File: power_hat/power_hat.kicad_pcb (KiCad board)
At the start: 4 copper layers, 47.1 x 133.6 mm, 49 parts, among them IC1 TPS259830LNRGER, IC2 INA238AQDGSRQ1, J1 XT30PW-M/Terminal block, J10 XT30PW-M/Terminal block, J11 XT30PW-M/Terminal block, J12 XT30PW-M/Terminal block, J13 502585-0570, J14 502585-0570, J2 XT30PW-M/Terminal block, J3 XT30PW-M/Terminal block, J4 XT30PW-M/Terminal block, J5 Conn_01x02_Pin, J6 XT30PW-M/Terminal block, J7 Conn_01x02_Pin, J8 XT30PW-M/Terminal block, J9 XT30PW-M/Terminal block, Q1 CSD18540Q5B

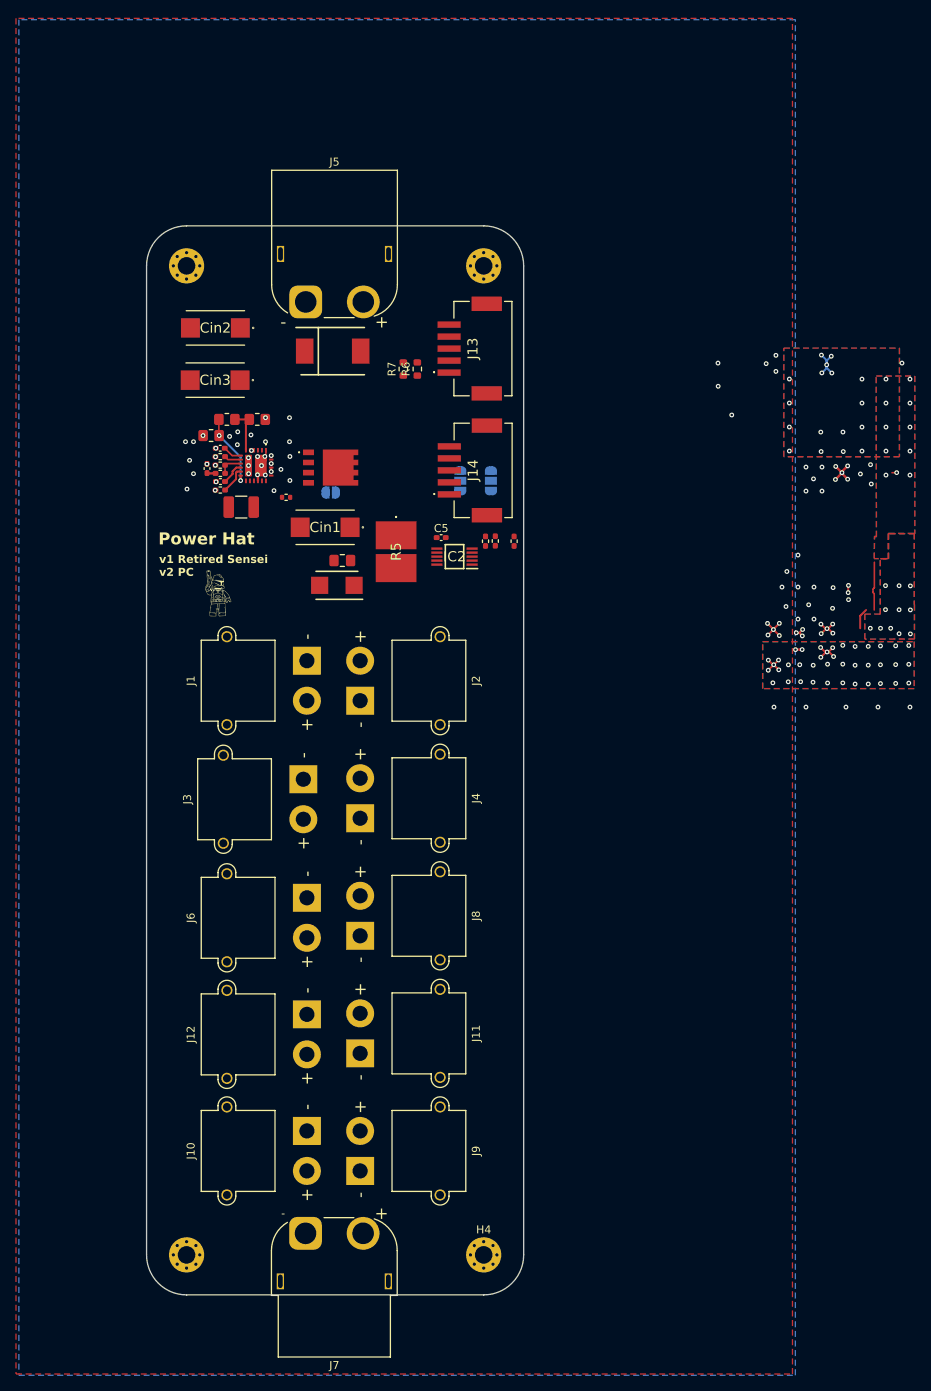
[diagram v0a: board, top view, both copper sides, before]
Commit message: Reruted a while ago with TPS, resized TPS with personal notes and Excel, issues with 24V one
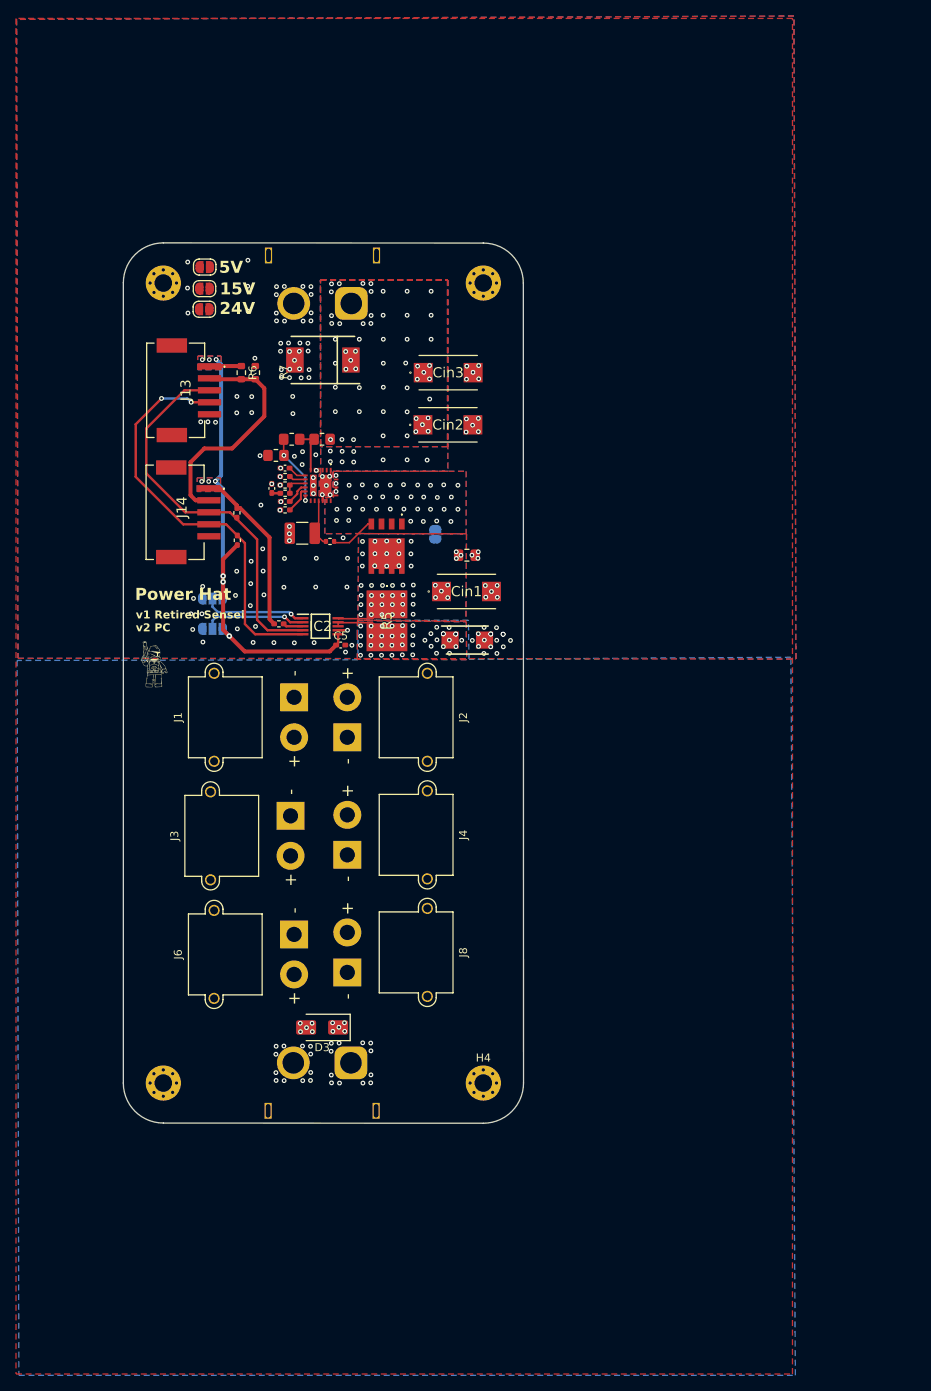
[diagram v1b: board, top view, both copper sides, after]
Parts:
- removed J10, J11, J12, J9: XT30PW-M/Terminal block, 0_connectors:AMASS_XT30PW-M_1x02_P2.50mm_Horizontal
- added D3: SMCJ28A, Diode_SMD:D_SMA, F.Cu at (83.2, 146.7)
- added JP4: Jumper_2_Open, Jumper:SolderJumper-2_P1.3mm_Open_RoundedPad1.0x1.5mm, F.Cu at (68.6, 51.6)
- added JP5: Jumper_2_Open, Jumper:SolderJumper-2_P1.3mm_Open_RoundedPad1.0x1.5mm, F.Cu at (68.5, 54.4)
- added JP6: Jumper_2_Open, Jumper:SolderJumper-2_P1.3mm_Open_RoundedPad1.0x1.5mm, F.Cu at (68.5, 56.9)
- J5, J7: moved to B.Cu
- moved J14 38.3 mm to (65.2, 82.3), turned to -90 degrees
- moved J13 38.2 mm to (65.2, 67.1), turned to -90 degrees
- moved JP3 37.8 mm to (69.5, 93.1), turned to 0 degrees
- moved JP2 36.1 mm to (69.5, 96.9), turned to 180 degrees
- moved R11 32.5 mm to (72.6, 82.4), turned to -90 degrees
- moved Cin2 31.5 mm to (99.0, 71.4), turned to 0 degrees
- moved R10 31.2 mm to (77.8, 96.2), turned to 180 degrees
- moved R12 31.0 mm to (72.7, 85.8), turned to 90 degrees
- moved Cin3 29.1 mm to (99.0, 64.8), turned to 0 degrees
- moved J7 22.1 mm to (86.8, 151.1), turned to 0 degrees
- moved R6 22.0 mm to (73.2, 64.8), turned to -90 degrees
- moved H2 21.7 mm to (63.4, 153.6)
- moved H4 21.5 mm to (103.4, 153.6)
- moved Cin1 19.4 mm to (101.3, 92.2), turned to 0 degrees
- moved IC2 18.9 mm to (83.0, 96.5), turned to 0 degrees
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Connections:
- IC2 pad 10: VCC -> /VOUT
- IC2 pad 8: /VOUT -> VCC
- IC2 pad 9: /VOUT -> VCC
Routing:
- net +3V3: track 0.00 -> 85.8 mm, vias 0 -> 9
- net /SCL: track 0.00 -> 52.3 mm, vias 0 -> 2
- net /SDA: track 0.00 -> 49.2 mm
- net /ID: track 0.00 -> 29.2 mm
- net GND: track 16.5 -> 2.54 mm, vias 72 -> 145
- net /A1: track 0.00 -> 13.0 mm, vias 0 -> 1
- net /A0: track 0.00 -> 12.8 mm, vias 0 -> 1
- net /VOUT: track 0.00 -> 6.86 mm, vias 0 -> 47
- net EFUSE: track 11.3 -> 5.38 mm, vias 37 -> 69
- net Net-(Q1-G): track 2.59 -> 5.69 mm
- net /ALERT: track 0.00 -> 2.53 mm
- net VCC: track 8.53 -> 7.38 mm, vias 39 -> 57
- net Net-(IC1-DVDT/_BGATE): track 6.10 -> 6.75 mm
- net /Efuse_out: vias 18 -> 36
- added copper zone on B.Cu, net +3V3
- added copper zone on F.Cu, net +3V3
- added copper zone on B.Cu, net /VOUT
- added copper zone on F.Cu, net /VOUT
- added copper zone on B.Cu, net GND
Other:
- board size 47.1 x 133.6 mm -> 50 x 110 mm
- board text added: "15V"
- board text added: "24V"
- board text added: "5V"
- board text added: "A0"
- board text added: "A1"
- board text added: "Address select"
- board text added: "Ok the Xt60 are put backwards because like this polarity is fixed"

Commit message: Rerouted and DRC repassed to put back ADM as TPS is thermally limited for 24V
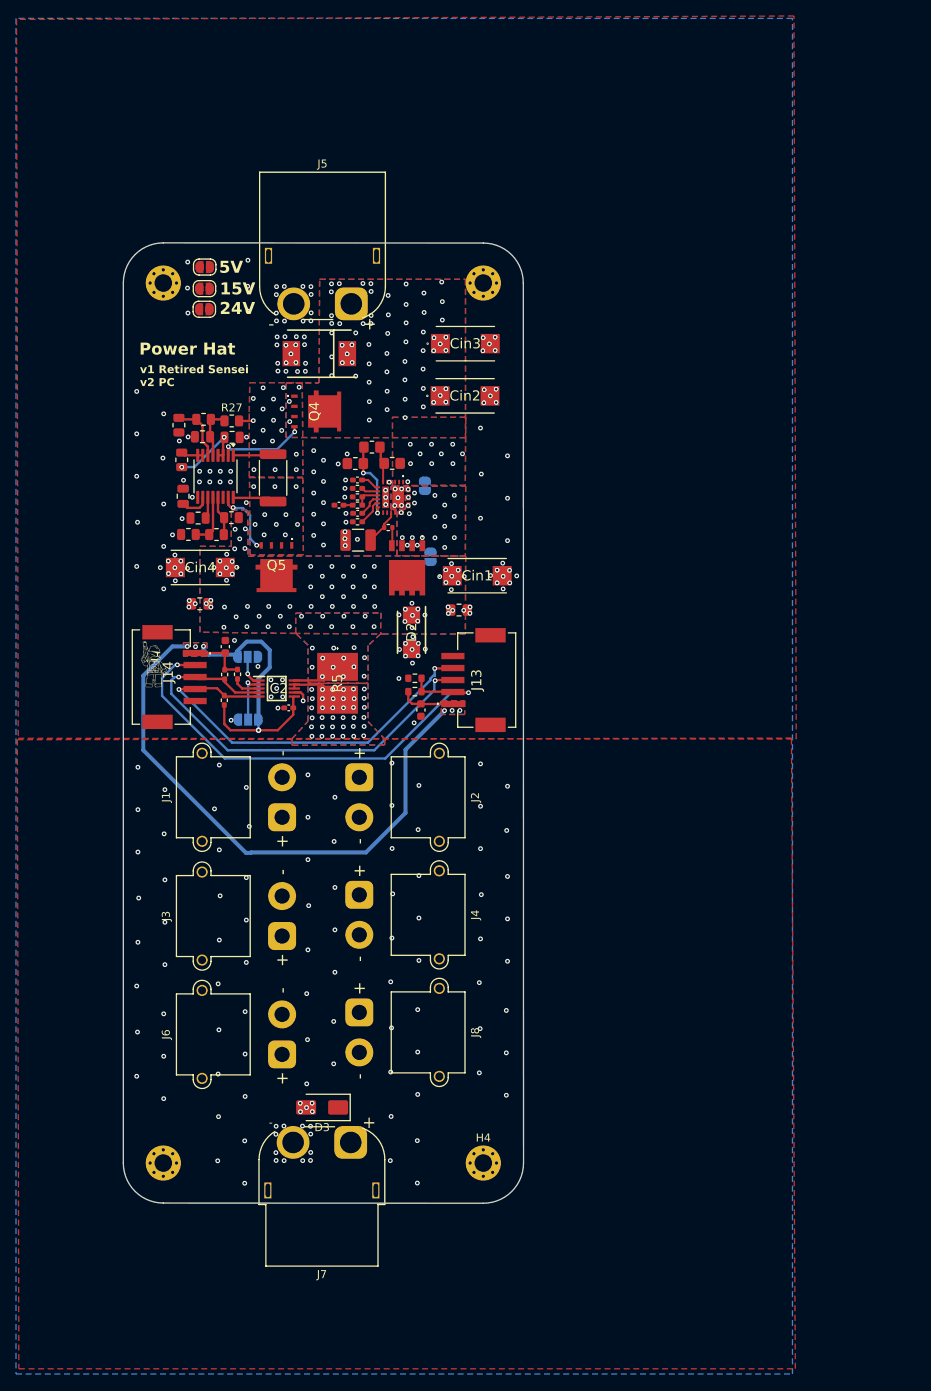
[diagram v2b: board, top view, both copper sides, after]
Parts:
- added C2: 1uF, Capacitor_SMD:C_0805_2012Metric_Pad1.18x1.45mm_HandSolder, F.Cu at (68.0, 93.7)
- added C3: 4u7 50V XR7, Capacitor_SMD:C_0603_1608Metric, F.Cu at (71.2, 99.1)
- added C38: 1uF - 50V X7R, Capacitor_SMD:C_0805_2012Metric, F.Cu at (72.0, 72.9)
- added C39: 1nF - 50V X7R, Capacitor_SMD:C_0805_2012Metric, F.Cu at (68.3, 72.9)
- added C4: 4u7 50V XR7, Capacitor_SMD:C_0603_1608Metric, F.Cu at (95.6, 107.0)
- added C40: 2.2uF, Capacitor_SMD:C_0805_2012Metric, F.Cu at (65.9, 80.3)
- added C41: 100nF - 50V X7R, Capacitor_SMD:C_0805_2012Metric, F.Cu at (67.8, 83.0)
- added Cin4: T521D475M063ATE075, lib_fp:T521D, F.Cu at (68.0, 89.2)
- added JP7: Jumper_2_Open, Jumper:SolderJumper-2_P1.3mm_Open_RoundedPad1.0x1.5mm, B.Cu at (96.1, 79.0)
- added Q4: SQJ461EP-T1_GE3, lib_fp:SQJ461EPT1_GE3, F.Cu at (82.6, 69.7)
- added Q5: SQJ461EP-T1_GE3, lib_fp:SQJ461EPT1_GE3, F.Cu at (77.5, 89.2)
- added R27: NOTE, Resistor_SMD:R_0805_2012Metric, F.Cu at (72.0, 70.9)
- added R28: NOTE, Resistor_SMD:R_0805_2012Metric, F.Cu at (68.4, 70.7)
- added R29: NOTE, Resistor_SMD:R_0805_2012Metric, F.Cu at (65.3, 71.4)
- added R32: 10k, Resistor_SMD:R_0805_2012Metric, F.Cu at (65.7, 75.8)
- added R33: 5m, Resistor_SMD:R_2512_6332Metric, F.Cu at (77.1, 78.0)
- added R34: 90k9, Resistor_SMD:R_0805_2012Metric, F.Cu at (71.9, 83.0)
- added R35: 174, Resistor_SMD:R_0805_2012Metric, F.Cu at (70.0, 85.1)
- added R36: 4k, Resistor_SMD:R_0805_2012Metric, F.Cu at (66.5, 85.1)
- added U17: ADM1270ARQZ, Package_SO:SSOP-16_3.9x4.9mm_P0.635mm, F.Cu at (69.9, 77.8)
- J1, J2, J3, J4, J6, J8: footprint 0_connectors:AMASS_XT30PW-M_1x02_P2.50mm_Horizontal -> Corrected_XT60:AMASS_XT30PW-M_1x02_P2.50mm_Horizontal
- J5: footprint Connector_AMASS:AMASS_XT60PW-M_1x02_P7.20mm_Horizontal -> Corrected_XT60:AMASS_XT60PW-M_1x02_P7.20mm_Horizontal; moved to F.Cu
- J7: footprint Connector_AMASS:AMASS_XT60PW-F_1x02_P7.20mm_Horizontal -> Corrected_XT60:AMASS_XT60PW-F_1x02_P7.20mm_Horizontal; moved to F.Cu
- moved J13 52.7 mm to (103.5, 103.3), turned to 90 degrees
- moved R6 45.4 mm to (94.8, 104.7), turned to 0 degrees
- moved R7 43.1 mm to (94.8, 103.0), turned to 0 degrees
- moved J14 20.7 mm to (63.5, 102.9)
- moved R11 20.3 mm to (71.1, 102.6)
- moved R12 20.1 mm to (71.0, 105.8)
- moved J7 12.3 mm to (79.6, 161.1), turned to 180 degrees
- moved JP2 12.2 mm to (74.0, 108.2)
- moved C5 10.2 mm to (79.1, 106.8), turned to 180 degrees
- moved J1 10.1 mm to (78.2, 115.4)
- moved J2 10.1 mm to (87.9, 120.4)
- moved J4 10.1 mm to (87.9, 135.1)
- moved J6 10.1 mm to (78.2, 145.1)
- moved J8 10.1 mm to (87.9, 149.8)
- moved J3 10.1 mm to (78.2, 130.3)
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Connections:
- C1 pad 1: /VOUT -> VOUT
- Cin1 pad 1: /VOUT -> VOUT
- D2 pad 1: VCC -> VOUT
- IC2 pad 10: /VOUT -> VOUT
- JP1 pad 2: /VOUT -> VOUT
- Q1 pad 5: /VOUT -> VOUT
- Q1 pad 6: /VOUT -> VOUT
- Q1 pad 7: /VOUT -> VOUT
- Q1 pad 8: /VOUT -> VOUT
- Q1 pad 9: /VOUT -> VOUT
- R5 pad 1: /VOUT -> VOUT
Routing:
- net +3V3: track 85.8 -> 121.5 mm, vias 9 -> 7
- net /ID: track 29.2 -> 59.6 mm, vias 0 -> 2
- net Net-(Q4-G): track 0.00 -> 11.1 mm, vias 0 -> 2
- net /VCAP: track 0.00 -> 9.85 mm, vias 0 -> 2
- net /A1: track 13.0 -> 3.99 mm
- net Net-(Q5-G): track 0.00 -> 8.88 mm, vias 0 -> 2
- net Net-(U17-OV): track 0.00 -> 7.35 mm
- net /SDA: track 49.2 -> 56.2 mm, vias 0 -> 2
- net /VOUT: track 6.86 -> 0.00 mm, vias 47 -> 0
- net /SENSE+: track 0.00 -> 6.85 mm, vias 0 -> 19
- net /A0: track 12.8 -> 6.13 mm
- net Net-(U17-FB_PG): track 0.00 -> 6.54 mm
- net Net-(U17-UV): track 0.00 -> 6.46 mm
- net VOUT: track 0.00 -> 6.11 mm, vias 0 -> 87
- net /SENSE-: track 0.00 -> 5.20 mm, vias 0 -> 10
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- added copper zone on B.Cu, net /SENSE+
- added copper zone on F.Cu, net /SENSE+
- added copper zone on B.Cu, net /SENSE-
- added copper zone on F.Cu, net /SENSE-
- added copper zone on B.Cu, net VOUT
- added copper zone on F.Cu, net VOUT
- removed copper zone on B.Cu, net /VOUT
- removed copper zone on F.Cu, net /VOUT
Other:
- board size 50 x 110 mm -> 50 x 120 mm
- board text added: "3V3"
- board text added: "GND"
- board text added: "U17"
- board text removed: "Ok the Xt60 are put backwards because like this polarity is fixed"
